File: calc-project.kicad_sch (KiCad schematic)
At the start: 54 parts, among them J2 Conn_01x08_Socket, J3 Conn_01x08_Socket, J4 Conn_01x08_Socket, SW1 SW_Push_45deg, SW10 SW_Push_45deg, SW11 SW_Push_45deg, SW12 SW_Push_45deg, SW13 SW_Push_45deg, SW14 SW_Push_45deg, SW15 SW_Push_45deg, SW16 SW_Push_45deg, SW17 SW_Push_45deg, SW18 SW_Push_45deg, SW19 SW_Push_45deg, SW2 SW_Push_45deg, SW20 SW_Push_45deg, SW21 SW_Push_45deg, SW22 SW_Push_45deg, SW23 SW_Push_45deg, SW24 SW_Push_45deg, SW25 SW_Push_45deg, SW26 SW_Push_45deg, SW27 SW_Push_45deg, SW28 SW_Push_45deg, SW29 SW_Push_45deg, SW3 SW_Push_45deg, SW30 SW_Push_45deg, SW31 SW_Push_45deg, SW32 SW_Push_45deg, SW33 SW_Push_45deg, SW34 SW_Push_45deg, SW35 SW_Push_45deg, SW36 SW_Push_45deg, SW37 SW_Push_45deg, SW38 SW_Push_45deg, SW39 SW_Push_45deg, SW4 SW_Push_45deg, SW40 SW_Push_45deg, SW41 SW_Push_45deg, SW42 SW_Push_45deg, SW43 SW_Push_45deg, SW44 SW_Push_45deg, SW45 SW_Push_45deg, SW46 SW_Push_45deg, SW47 SW_Push_45deg, SW48 SW_Push_45deg, SW5 SW_Push_45deg, SW6 SW_Push_45deg, SW7 SW_Push_45deg, SW8 SW_Push_45deg, SW9 SW_Push_45deg

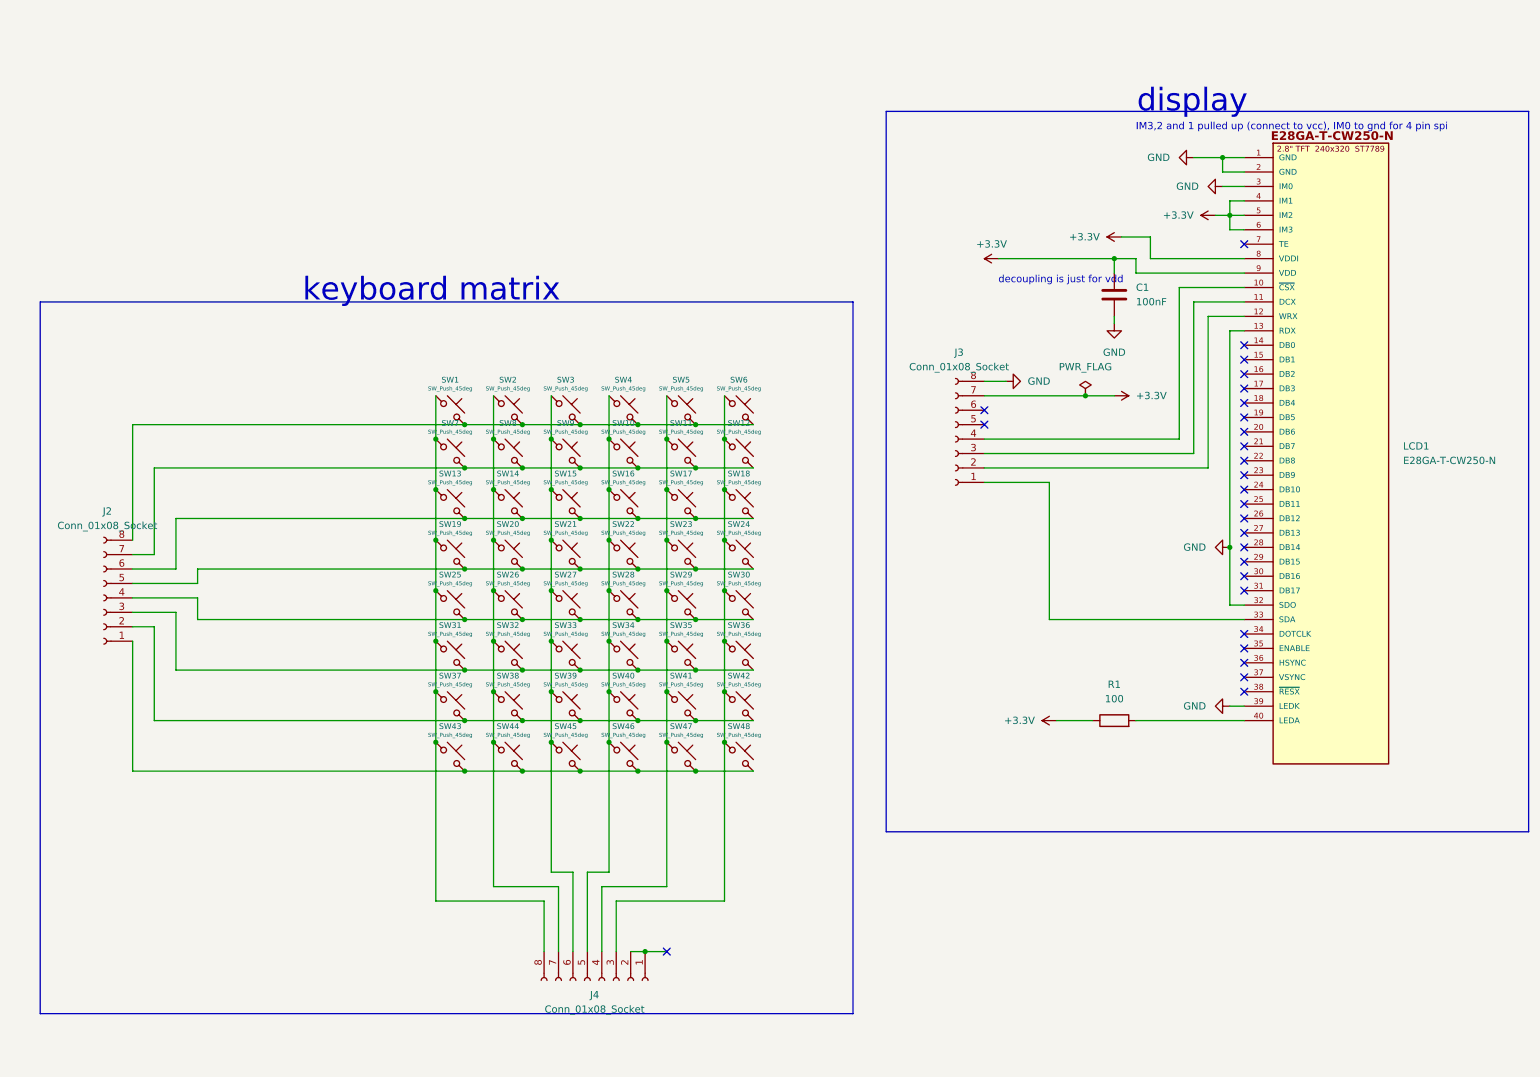
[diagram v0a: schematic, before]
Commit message: added rpi pico, took away connectors, idk what else
idk what i did
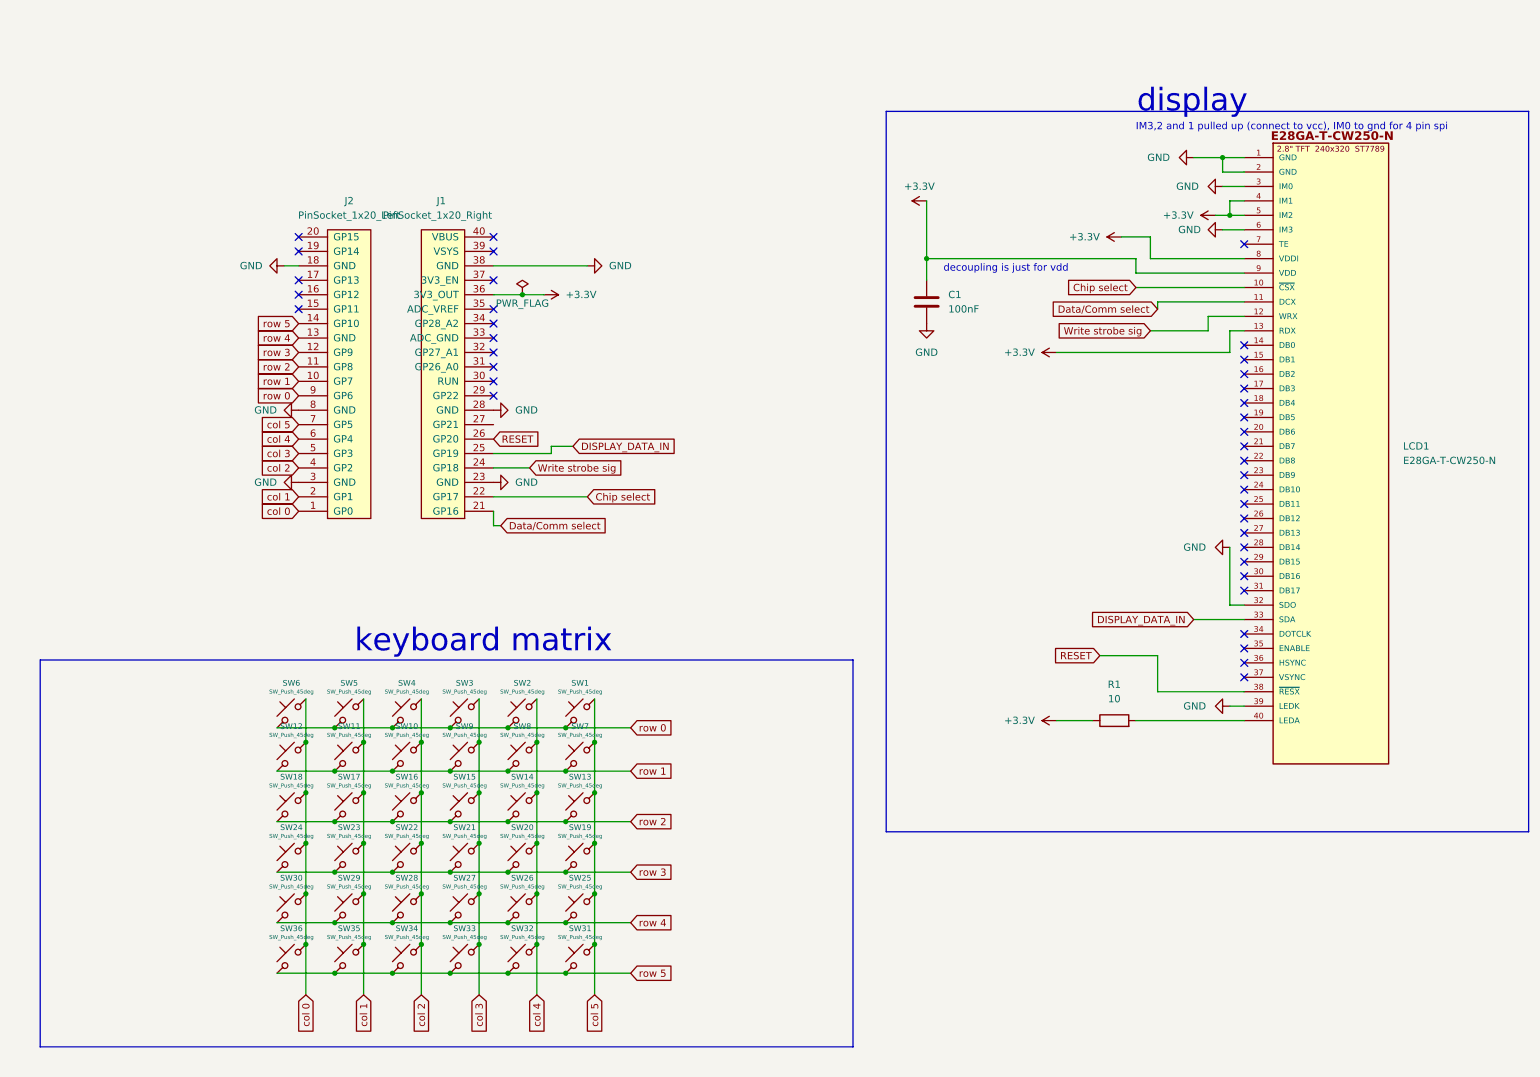
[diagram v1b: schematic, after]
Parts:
- removed J2, J3, J4: Conn_01x08_Socket, Connector_PinSocket_1.00mm:PinSocket_1x08_P1.00mm_Vertical, symbol Connector:Conn_01x08_Socket
- removed SW37, SW38, SW39, SW40, SW41, SW42, SW43, SW44, SW45, SW46, SW47, SW48: SW_Push_45deg, Library:SW_TL3315NF160Q, symbol Switch:SW_Push_45deg
- added J1: PinSocket_1x20_Right, Connector_PinSocket_2.54mm:PinSocket_1x20_P2.54mm_Vertical_SMD_Pin1Left, symbol Custom parts:PinSocket_1x20_Right
- added J2: PinSocket_1x20_Left, Connector_PinSocket_2.54mm:PinSocket_1x20_P2.54mm_Vertical_SMD_Pin1Left, symbol Custom parts:PinSocket_1x20_Left
- R1: value 100 -> 10
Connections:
- net +3.3V: now also LCD1.13 (RDX), J1.36 (3V3_OUT); no longer LCD1.6 (IM3)
- net GND: now also LCD1.6 (IM3), J1.23 (GND), J1.28 (GND), J1.38 (GND), J2.18 (GND), J2.3 (GND), J2.8 (GND); no longer LCD1.13 (RDX)
- net col 2: now reaches SW10.1, SW16.1, SW22.1, SW28.1, SW34.1, SW4.1
- net col 2: now also J2.4 (GP2)
- net row 0: now reaches SW1.2, SW2.2, SW3.2, SW4.2, SW5.2, SW6.2
- net row 0: now also J2.9 (GP6)
- net col 0: now reaches SW12.1, SW18.1, SW24.1, SW30.1, SW36.1, SW6.1
- net col 0: now also J2.1 (GP0)
- net col 4: now reaches SW14.1, SW2.1, SW20.1, SW26.1, SW32.1, SW8.1
- net col 4: now also J2.6 (GP4)
- net row 4: now reaches SW25.2, SW26.2, SW27.2, SW28.2, SW29.2, SW30.2
- net row 4: now also J2.13 (GND)
- net DISPLAY_DATA_IN: now reaches LCD1.33 (SDA)
- net DISPLAY_DATA_IN: now also J1.25 (GP19)
- net Write strobe sig: now reaches LCD1.12 (WRX)
- net Write strobe sig: now also J1.24 (GP18)
- net Data/Comm select: now reaches LCD1.11 (DCX)
- net Data/Comm select: now also J1.21 (GP16)
- net Chip select: now reaches LCD1.10 (~{CSX})
- net Chip select: now also J1.22 (GP17)
- net col 1: now reaches SW11.1, SW17.1, SW23.1, SW29.1, SW35.1, SW5.1
- net col 1: now also J2.2 (GP1)
- net row 1: now reaches SW10.2, SW11.2, SW12.2, SW7.2, SW8.2, SW9.2
- net row 1: now also J2.10 (GP7)
- net row 3: now reaches SW19.2, SW20.2, SW21.2, SW22.2, SW23.2, SW24.2
- net row 3: now also J2.12 (GP9)
- net col 5: now reaches SW1.1, SW13.1, SW19.1, SW25.1, SW31.1, SW7.1
- net col 5: now also J2.7 (GP5)
- net row 5: now reaches SW31.2, SW32.2, SW33.2, SW34.2, SW35.2, SW36.2
- net row 5: now also J2.14 (GP10)
- net col 3: now reaches SW15.1, SW21.1, SW27.1, SW3.1, SW33.1, SW9.1
- net col 3: now also J2.5 (GP3)
- net row 2: now reaches SW13.2, SW14.2, SW15.2, SW16.2, SW17.2, SW18.2
- net row 2: now also J2.11 (GP8)
- net RESET: now reaches LCD1.38 (~{RESX})
- net RESET: now also J1.26 (GP20)
- no-connect marks 27 -> 38
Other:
- moved on the sheet: C1, SW1, SW10, SW11, SW12, SW13, SW14, SW15, SW16, SW17, SW18, SW19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

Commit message: idek if this is progress or not
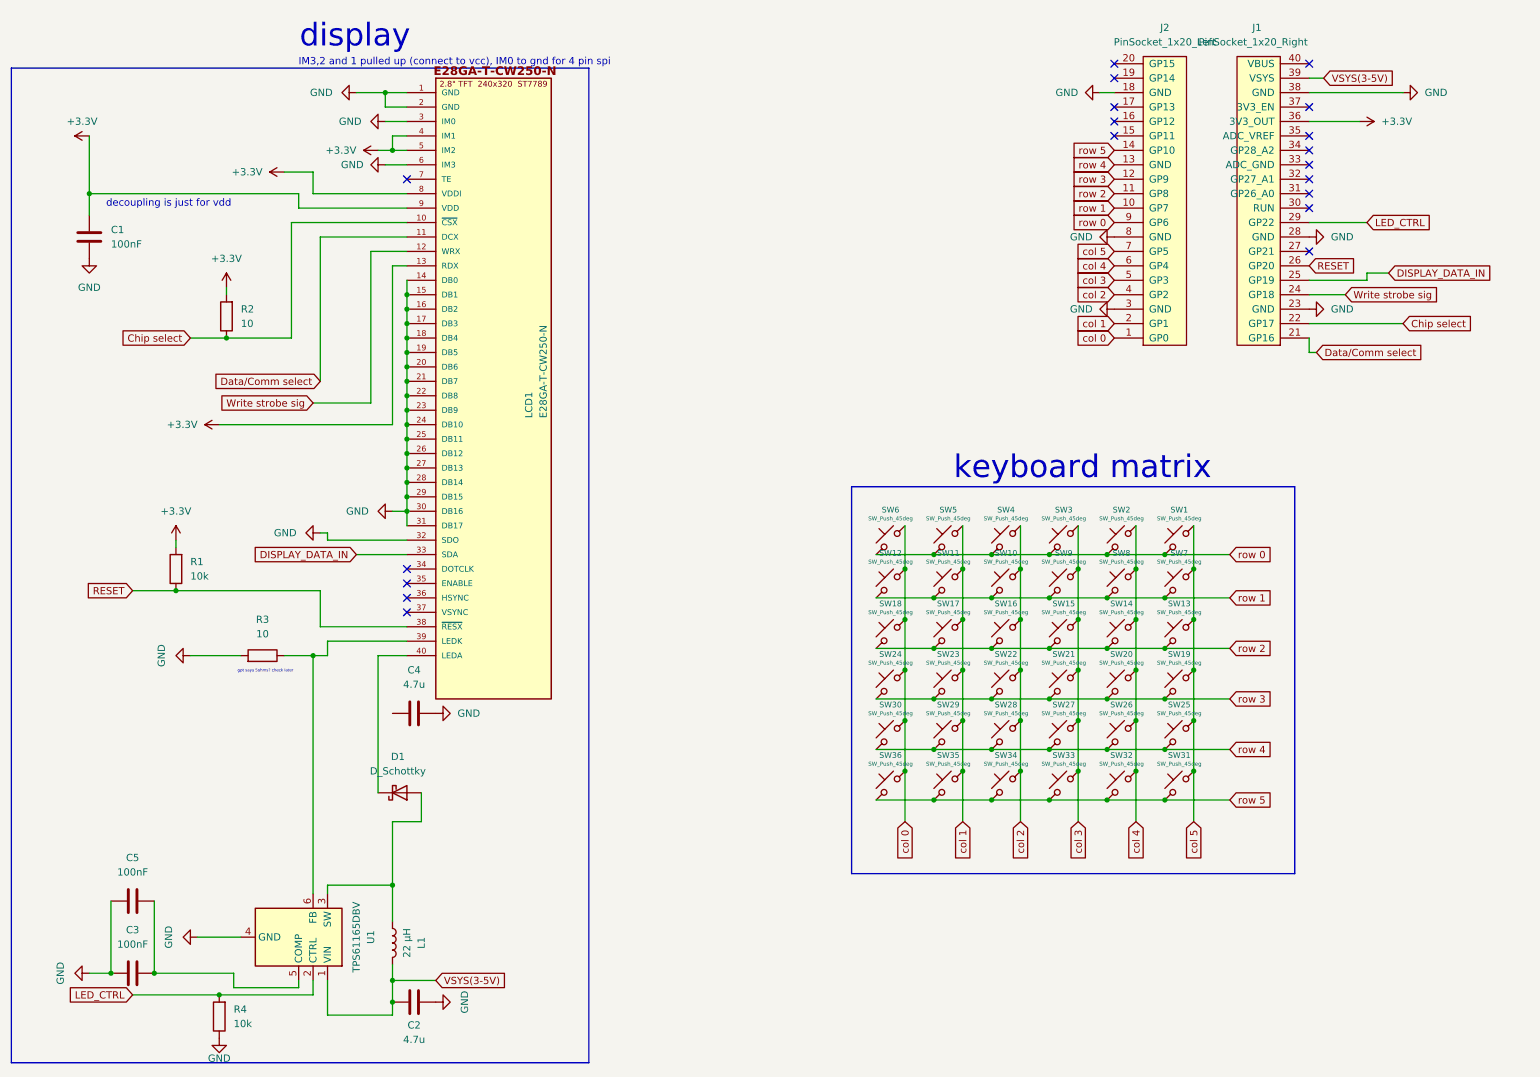
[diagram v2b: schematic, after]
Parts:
- added C2, C4: 4.7u, Capacitor_SMD:C_0201_0603Metric_Pad0.64x0.40mm_HandSolder, symbol Device:C
- added C3, C5: 100nF, Capacitor_SMD:C_0201_0603Metric_Pad0.64x0.40mm_HandSolder, symbol Device:C
- added D1: D_Schottky, symbol Device:D_Schottky
- added L1: 22 µH, symbol Device:L
- added R2, R3: 10, Resistor_SMD:R_0201_0603Metric_Pad0.64x0.40mm_HandSolder, symbol Device:R
- added R4: 10k, Resistor_SMD:R_0201_0603Metric_Pad0.64x0.40mm_HandSolder, symbol Device:R
- added U1: TPS61165DBV, Package_TO_SOT_SMD:SOT-23-6, symbol Driver_LED:TPS61165DBV
- R1: value 10 -> 10k
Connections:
- net +3.3V: now also R1.2, R2.2; no longer R1.1
- net Chip select: now also R2.1
- net GND: now also LCD1.14 (DB0), LCD1.15 (DB1), LCD1.16 (DB2), LCD1.17 (DB3), LCD1.18 (DB4), LCD1.19 (DB5), LCD1.20 (DB6), LCD1.21 (DB7), LCD1.22 (DB8), LCD1.23 (DB9), LCD1.24 (DB10), LCD1.25 (DB11), LCD1.26 (DB12), LCD1.27 (DB13), LCD1.28 (DB14), LCD1.29 (DB15), LCD1.30 (DB16), LCD1.31 (DB17), C2.1, C3.1, C4.2, C5.1, R3.2, R4.1, U1.4 (GND); no longer LCD1.39 (LEDK)
- net RESET: now also R1.1
- net at LCD1.40 (LEDA): now also D1.1 (K); no longer R1.2
- net LED_CTRL: now reaches J1.29 (GP22)
- net LED_CTRL: now also R4.2, U1.2 (CTRL)
- net VSYS(3-5V): now reaches J1.39 (VSYS)
- net VSYS(3-5V): now also C2.2, L1.1, U1.1 (VIN)
- new net: C3.2, C5.2, U1.5 (COMP)
- new net: D1.2 (A), L1.2, U1.3 (SW)
- new net: LCD1.39 (LEDK), R3.1, U1.6 (FB)
- no-connect marks 38 -> 19
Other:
- note added: "gpt says 5ohms? check later"
- moved on the sheet: C1, LCD1
